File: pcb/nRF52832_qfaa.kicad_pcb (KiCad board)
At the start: 4 copper layers, 41.5 x 13 mm, 75 parts, among them J1 Conn_01x01_Female, J2 Conn_02x05_Odd_Even, U1 NRF52832, U2 W25Q32JVZP, U3 TPS63802DLAR, U4 BQ24078RGTR, U5 RV-4162-C7, U6 SN74LVC1G79DBVT, X1 32.768kHz, X2 32MHz

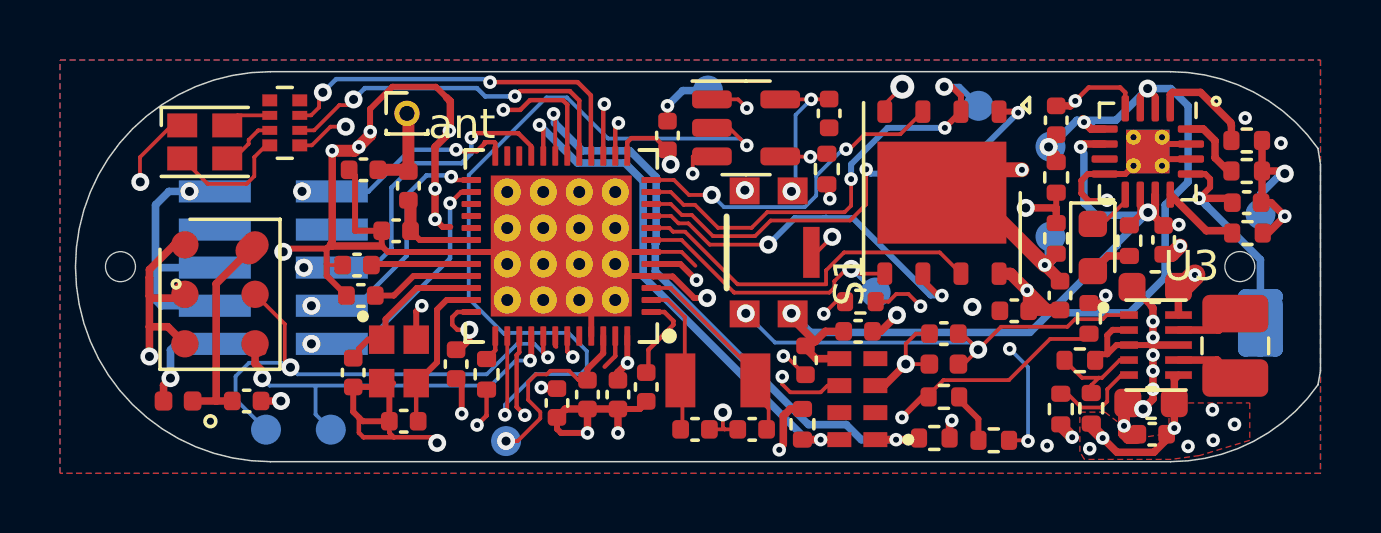
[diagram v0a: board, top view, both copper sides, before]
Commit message: [pcb] finalized layout of v1.3
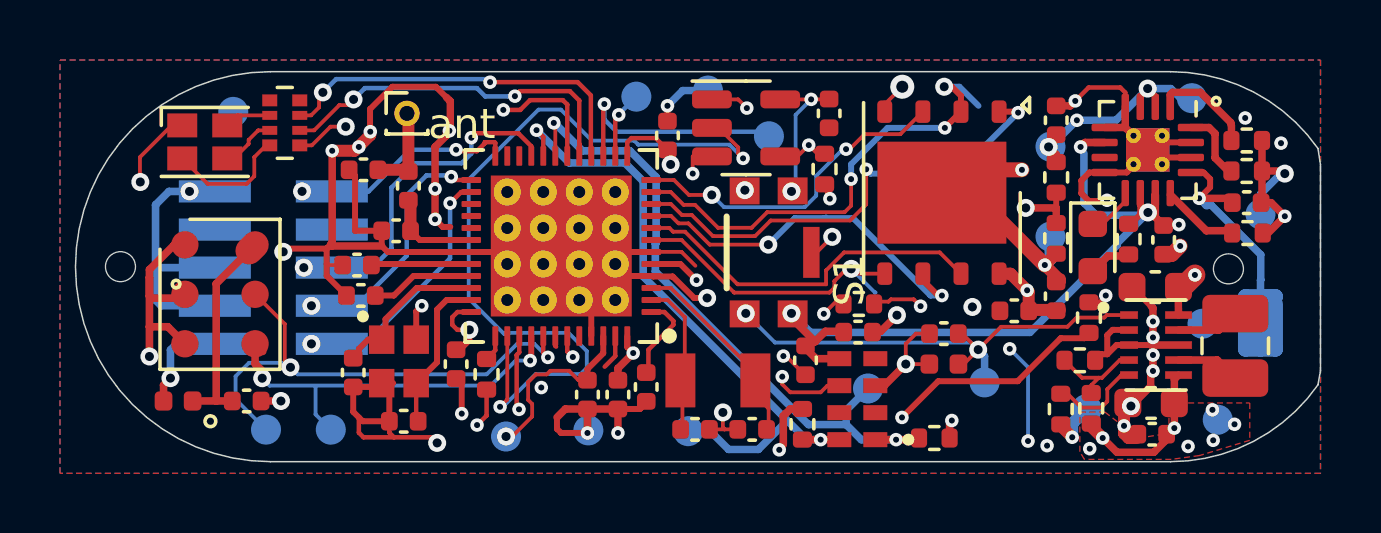
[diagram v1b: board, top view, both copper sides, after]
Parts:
- removed the C2 at (45.5, 39.9)
- removed the R5 at (58.4, 39.7)
- removed R_DNP_1: 1.6K, Resistor_SMD:R_0402_1005Metric
- removed TP12, TP14: TestPoint, TestPoint:TestPoint_Pad_D1.0mm
- added TP16: TestPoint, TestPoint:TestPoint_Pad_D1.0mm, B.Cu at (59.8, 39.2)
- added TP18: TestPoint, TestPoint:TestPoint_Pad_D1.0mm, B.Cu at (55.9, 39.4)
- added TP19: TestPoint, TestPoint:TestPoint_Pad_D1.0mm, B.Cu at (34.7, 30.2)
- added TP24: TestPoint, TestPoint:TestPoint_Pad_D1.0mm, B.Cu at (63.2, 40.1)
- added TP25: TestPoint, TestPoint:TestPoint_Pad_D1.0mm, B.Cu at (67.5, 40.4)
- added TP26: TestPoint, TestPoint:TestPoint_Pad_D1.0mm, B.Cu at (67.0, 37.2)
- added TP27: TestPoint, TestPoint:TestPoint_Pad_D1.0mm, B.Cu at (66.7, 29.7)
- added TP28: TestPoint, TestPoint:TestPoint_Pad_D1.0mm, B.Cu at (46.6, 40.8)
- added TP5: TestPoint, TestPoint:TestPoint_Pad_D1.0mm, B.Cu at (49.9, 40.8)
- added TP6: TestPoint, TestPoint:TestPoint_Pad_D1.0mm, B.Cu at (52.6, 31.0)
- added TP7: TestPoint, TestPoint:TestPoint_Pad_D1.0mm, B.Cu at (48.2, 29.7)
- moved H1 0.39 mm to (67.9, 35.4)
- moved TP11 0.15 mm to (43.8, 41.0)
- moved C17 0.13 mm to (62.2, 36.3)
- moved R12 0.09 mm to (55.6, 36.6)
- moved R17 0.08 mm to (54.4, 32.1)
- moved R9 0.06 mm to (64.6, 34.4)
- moved U4 0.05 mm to (65.2, 31.4)
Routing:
- net +BATT: track 19.2 -> 8.34 mm
- net /P0.12: track 1.75 -> 7.98 mm
- net /I2C_SCL: track 17.9 -> 21.9 mm
- net V_charger: track 14.4 -> 16.5 mm
- net VSS: track 49.1 -> 51.1 mm
- net /Power/LDO_EN: track 2.01 -> 0.00 mm
- net MAIN_BUTTON: track 31.7 -> 33.1 mm
- net GND: track 127.7 -> 129.1 mm, vias 41 -> 40
- net /P0.11: track 1.15 -> 2.27 mm
- net /I2C_SDA: track 20.9 -> 21.8 mm
- net VCC: track 90.0 -> 89.2 mm
- net FF_CLK: track 28.1 -> 27.5 mm
- net MCU_POWER_LATCH: track 23.0 -> 23.5 mm
- net /DEC4: track 6.97 -> 6.46 mm
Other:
- board text removed: "gnd"
- board text removed: "rx"
- board text removed: "tx"
